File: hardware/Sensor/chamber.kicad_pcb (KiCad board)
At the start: 2 copper layers, 45 x 30 mm, 34 parts, among them U10 LMC662, U11 LM358, U20 ICL7660

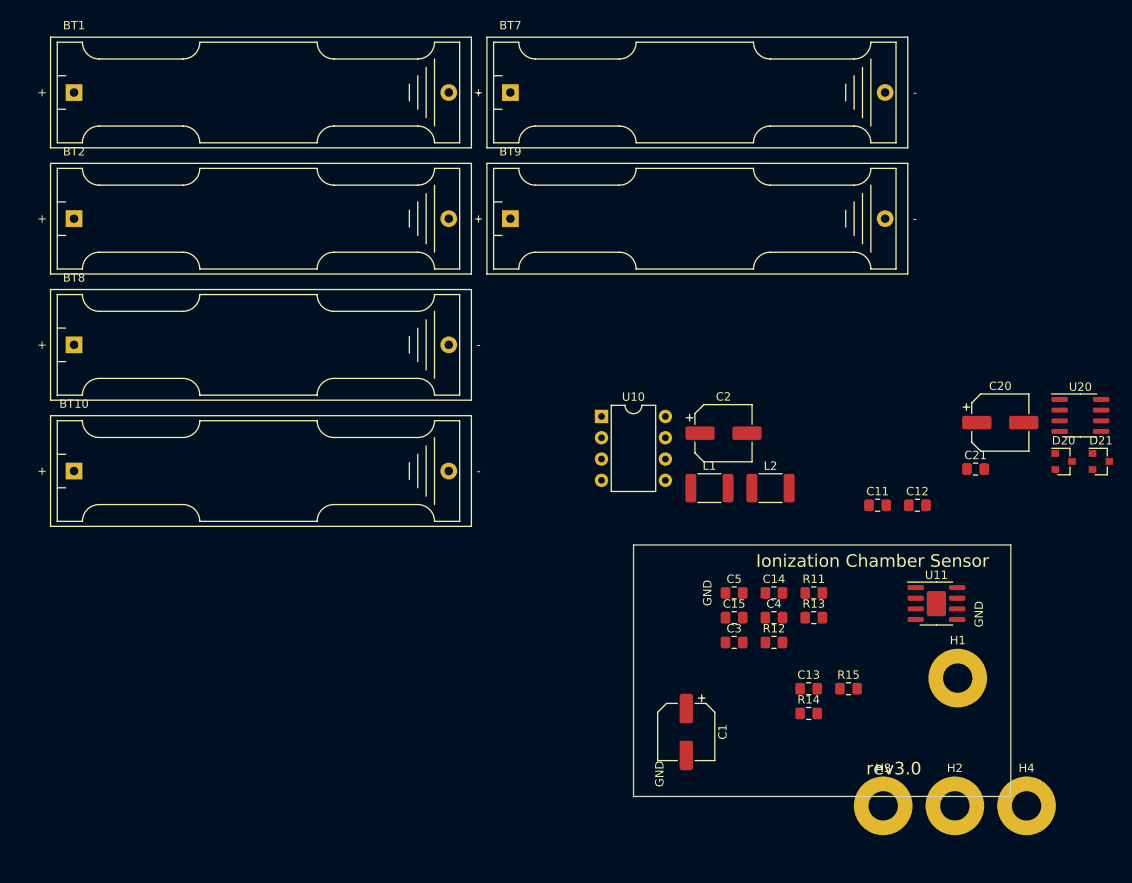
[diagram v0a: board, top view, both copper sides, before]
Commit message: sensor + high voltage schemat
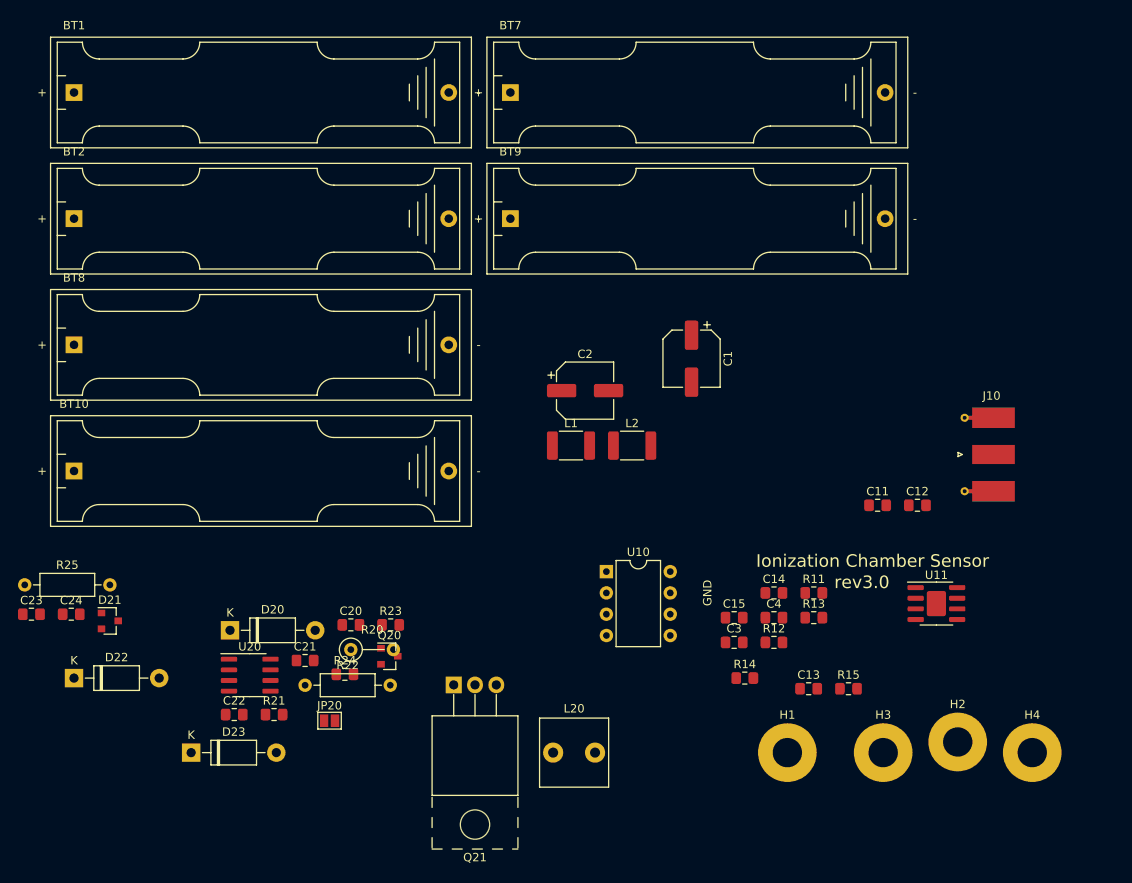
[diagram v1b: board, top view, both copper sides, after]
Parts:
- removed C5: 100n, Capacitor_SMD:C_0805_2012Metric_Pad1.15x1.40mm_HandSolder
- added C22: 10n, Capacitor_SMD:C_0805_2012Metric_Pad1.15x1.40mm_HandSolder, F.Cu at (67.4, 60.2)
- added C23: 10n/600V, Capacitor_SMD:C_0805_2012Metric_Pad1.15x1.40mm_HandSolder, F.Cu at (43.2, 48.3)
- added C24: 10n/600V, Capacitor_SMD:C_0805_2012Metric_Pad1.15x1.40mm_HandSolder, F.Cu at (47.9, 48.3)
- added D22: 1N4007, Diode_THT:D_DO-41_SOD81_P10.16mm_Horizontal, F.Cu at (48.3, 55.9)
- added D23: 1N4007, Diode_THT:D_DO-41_SOD81_P10.16mm_Horizontal, F.Cu at (62.2, 64.8)
- added J10: Conn_Coaxial, Connector_Coaxial:SMA_Molex_73251-1153_EdgeMount_Horizontal, F.Cu at (156.2, 29.2)
- added JP20: close(1) = disable HV gen, Jumper:SolderJumper-2_P1.3mm_Open_Pad1.0x1.5mm, F.Cu at (78.7, 61.0)
- added L20: 680m, Inductor_THT:L_Radial_L8.0mm_W8.0mm_P5.00mm_Neosid_NE-CPB-07E, F.Cu at (105.4, 64.8)
- added Q20: BC859, Package_TO_SOT_SMD:SOT-23, F.Cu at (85.9, 53.3)
- added Q21: Q_NMOS_GDS, Package_TO_SOT_THT:TO-220-3_Horizontal_TabUp, F.Cu at (93.5, 56.7)
- added R20: R22/0.5W, Resistor_THT:R_Axial_DIN0207_L6.3mm_D2.5mm_P5.08mm_Vertical, F.Cu at (81.3, 52.5)
- added R21: 10k, Resistor_SMD:R_0805_2012Metric_Pad1.15x1.40mm_HandSolder, F.Cu at (72.1, 60.2)
- added R22: 10M, Resistor_THT:R_Axial_DIN0207_L6.3mm_D2.5mm_P10.16mm_Horizontal, F.Cu at (75.8, 56.7)
- added R23: 1k, Resistor_SMD:R_0805_2012Metric_Pad1.15x1.40mm_HandSolder, F.Cu at (86.0, 49.5)
- added R24: 30k, Resistor_SMD:R_0805_2012Metric_Pad1.15x1.40mm_HandSolder, F.Cu at (80.6, 55.4)
- added R25: 10M, Resistor_THT:R_Axial_DIN0207_L6.3mm_D2.5mm_P10.16mm_Horizontal, F.Cu at (42.4, 44.8)
- C20: value 10u/16V -> 3n2; footprint Capacitor_SMD:CP_Elec_6.3x5.4 -> Capacitor_SMD:C_0805_2012Metric_Pad1.15x1.40mm_HandSolder
- D20: value D_Schottky -> 1N4007; footprint Diode_SMD:D_SOT-23_ANK -> Diode_THT:D_DO-41_SOD81_P10.16mm_Horizontal
- U20: value ICL7660 -> MC34063AD
- moved D21 119.7 mm to (52.5, 49.1)
- moved U20 103.8 mm to (69.2, 55.5)
- moved D20 101.4 mm to (66.9, 50.2)
- moved C21 83.2 mm to (75.8, 53.8)
- moved C20 81.1 mm to (81.3, 49.5)
- moved C1 44.5 mm to (121.9, 17.8)
- moved H1 22.2 mm to (133.3, 64.8)
- moved U10 18.5 mm to (111.8, 43.2)
- moved C2 17.3 mm to (109.2, 21.6)
- moved L2 17.3 mm to (114.8, 28.1)
- moved L1 17.3 mm to (107.5, 28.1)
- moved R14 8.71 mm to (128.3, 55.9)
- moved H2 7.63 mm to (153.7, 63.5)
- moved H4 6.39 mm to (162.6, 64.8)
- moved H3 6.35 mm to (144.8, 64.8)
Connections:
- C20 pad 2: Net-(C20-Pad2) -> GND
- C21 pad 1: (no net) -> GND
- C21 pad 2: (no net) -> +BATT
- D20 pad 1: Net-(C20-Pad2) -> Net-(C23-Pad1)
- D21 pad 1: (no net) -> Net-(D21-Pad1)
- D21 pad 2: (no net) -> Net-(D21-Pad2)
- U20 pad 1: (no net) -> Net-(L20-Pad1)
- U20 pad 2: Net-(C20-Pad1) -> Net-(D21-Pad2)
- U20 pad 3: -BATT -> Net-(C20-Pad1)
- U20 pad 4: (no net) -> GND
- U20 pad 5: -BATT -> Net-(C22-Pad1)
- U20 pad 6: (no net) -> +BATT
- U20 pad 7: (no net) -> Net-(L20-Pad1)
- U20 pad 8: Net-(D20-Pad2) -> Net-(L20-Pad1)
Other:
- board outline removed
